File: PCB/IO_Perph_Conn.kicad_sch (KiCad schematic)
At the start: 1 part, among them U2 STM32MP157FABx

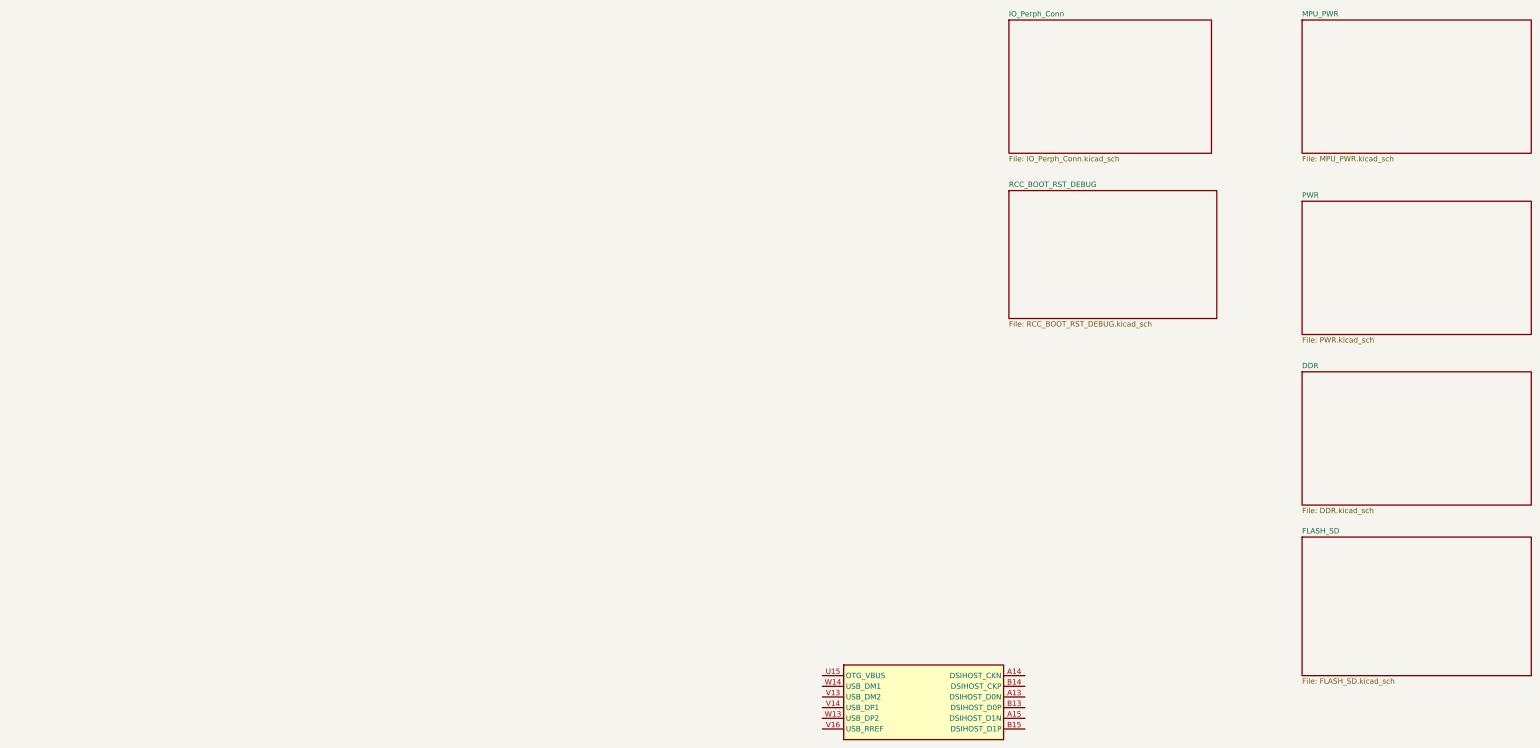
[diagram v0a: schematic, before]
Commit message: PCB_UPDATE
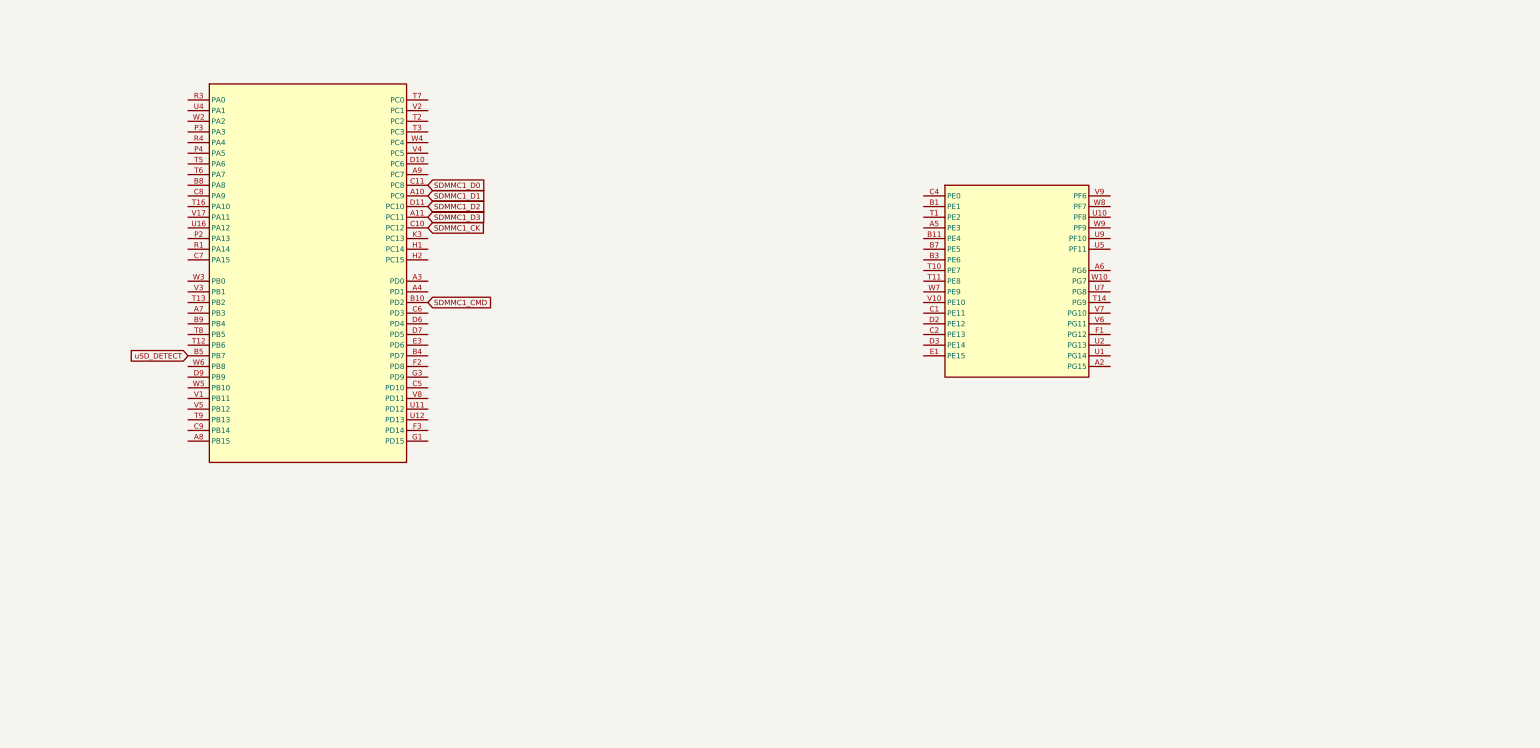
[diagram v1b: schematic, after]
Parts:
- removed U2: STM32MP157FABx, Package_BGA:ST_LFBGA-354_16x16mm_Layout19x19_P0.8mm, symbol New_Library:STM32MP157FABx
- added U2: STM32MP157FABx, Package_BGA:ST_LFBGA-354_16x16mm_Layout19x19_P0.8mm, symbol New_Library:STM32MP157FABx
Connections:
- new net SDMMC1_CK: U2.C10 (PC12)
- new net SDMMC1_CMD: U2.B10 (PD2)
- new net SDMMC1_D0: U2.C11 (PC8)
- new net SDMMC1_D1: U2.A10 (PC9)
- new net SDMMC1_D2: U2.D11 (PC10)
- new net SDMMC1_D3: U2.A11 (PC11)
- new net uSD_DETECT: U2.B5 (PB7)
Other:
- removed sheet DDR
- removed sheet FLASH_SD
- removed sheet IO_Perph_Conn
- removed sheet MPU_PWR
- removed sheet PWR
- removed sheet RCC_BOOT_RST_DEBUG

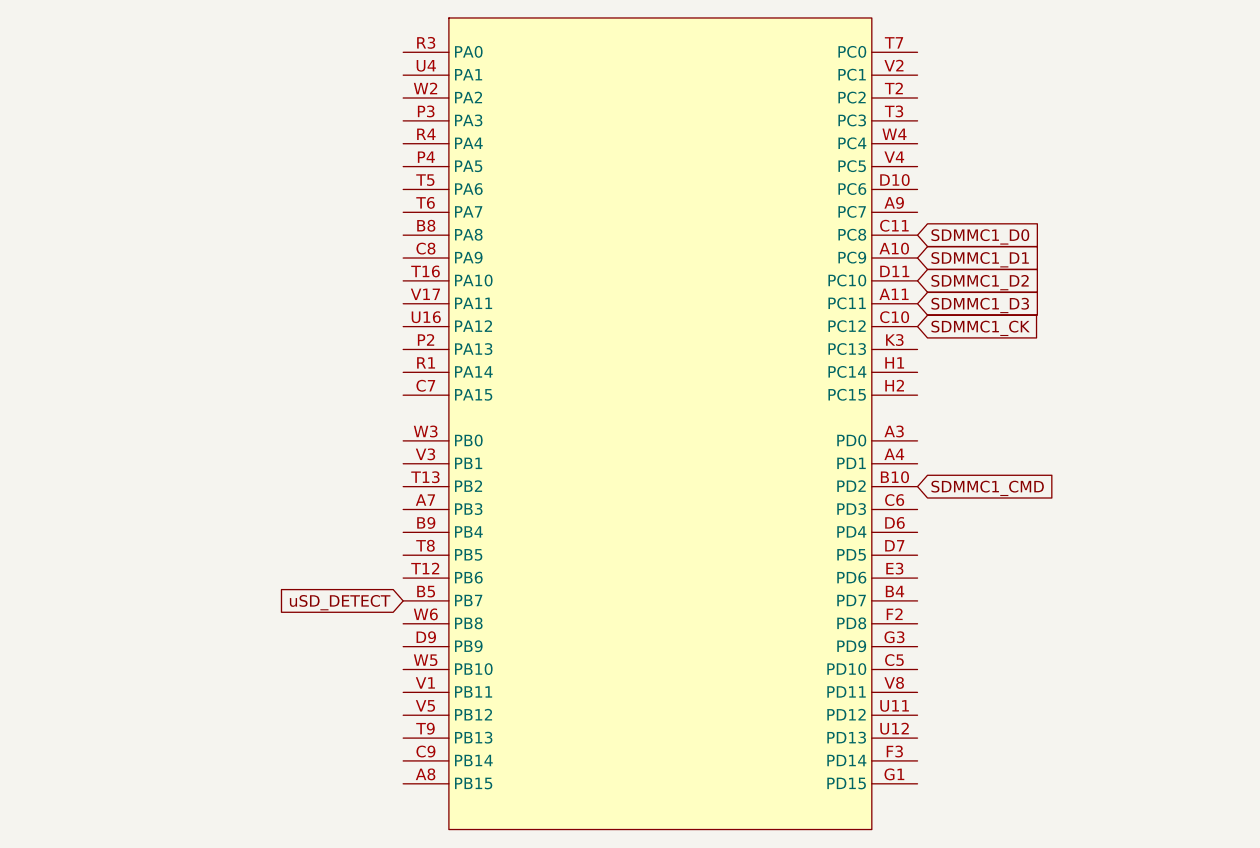
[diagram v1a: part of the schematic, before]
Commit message: Look like MPU done
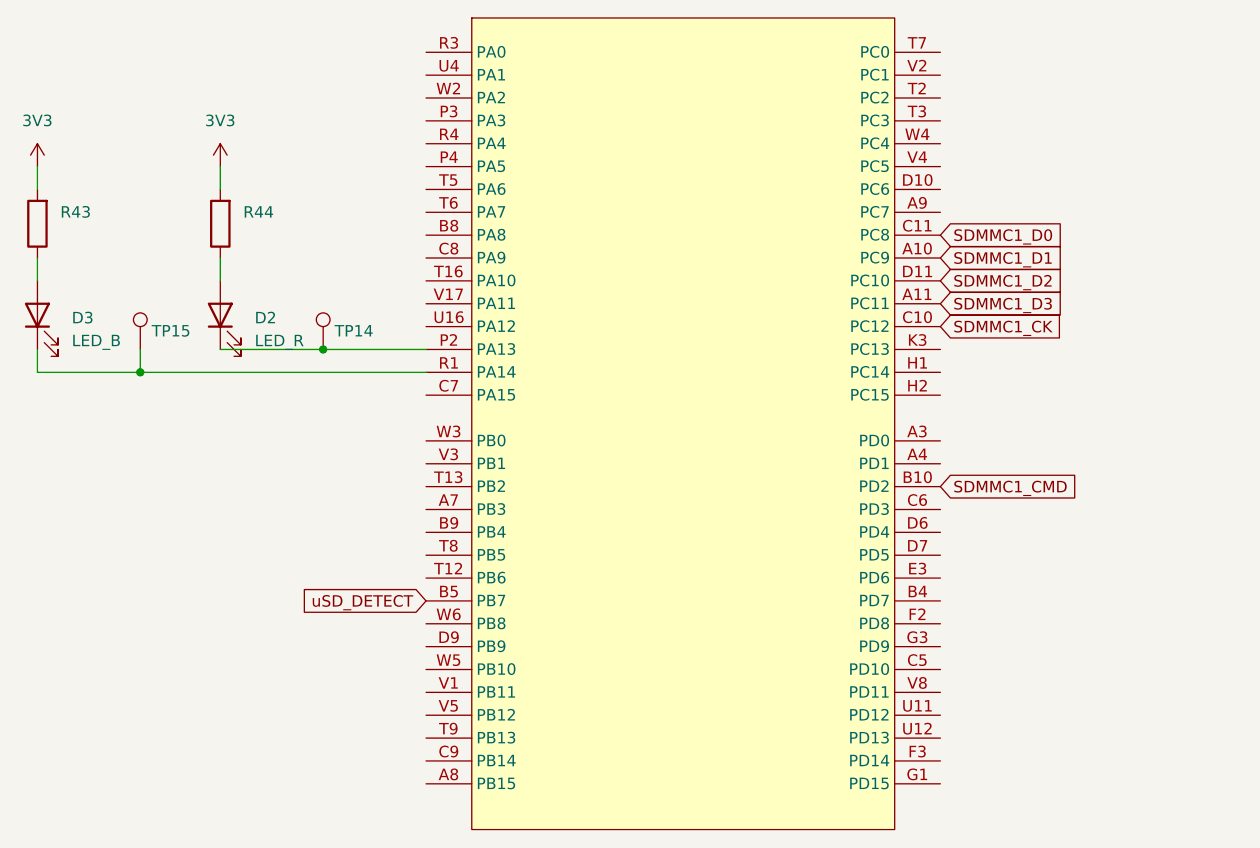
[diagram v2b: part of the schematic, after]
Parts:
- added D2: LED_R, LED_SMD:LED_0402_1005Metric, symbol Device:LED
- added D3: LED_B, LED_SMD:LED_0402_1005Metric, symbol Device:LED
- added R43, R44: ~, symbol Device:R
- added TP14, TP15: TestPoint, TestPoint:TestPoint_Pad_D1.0mm, symbol Connector:TestPoint
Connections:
- net at U2.P2 (PA13): now also D2.1 (K), TP14.1
- net at U2.R1 (PA14): now also D3.1 (K), TP15.1
- new net: D3.2 (A), R43.1
- new net: D2.2 (A), R44.1
- new net 3V3: R43.2, R44.2
